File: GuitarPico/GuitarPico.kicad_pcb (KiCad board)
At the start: 2 copper layers, 100 x 100 mm, 132 parts, among them J1 INPUT, J2 INPUT, J3 OUTPUT, J4 OUTPUT, J5 Barrel_Jack_Switch, J6 VGA, J8 INPUT, J9 INPUT, Q1 2N3904, Q2 2N3904, Q3 2N3904, SW1 SW_Push, SW2 SW_Push, SW3 SW_Push, SW4 SW_Push, SW5 SW_Push, U1 LM358, U2 LM358, U3 Pico, U4 LM7805_TO220, U5 TL431LP, U6 4051

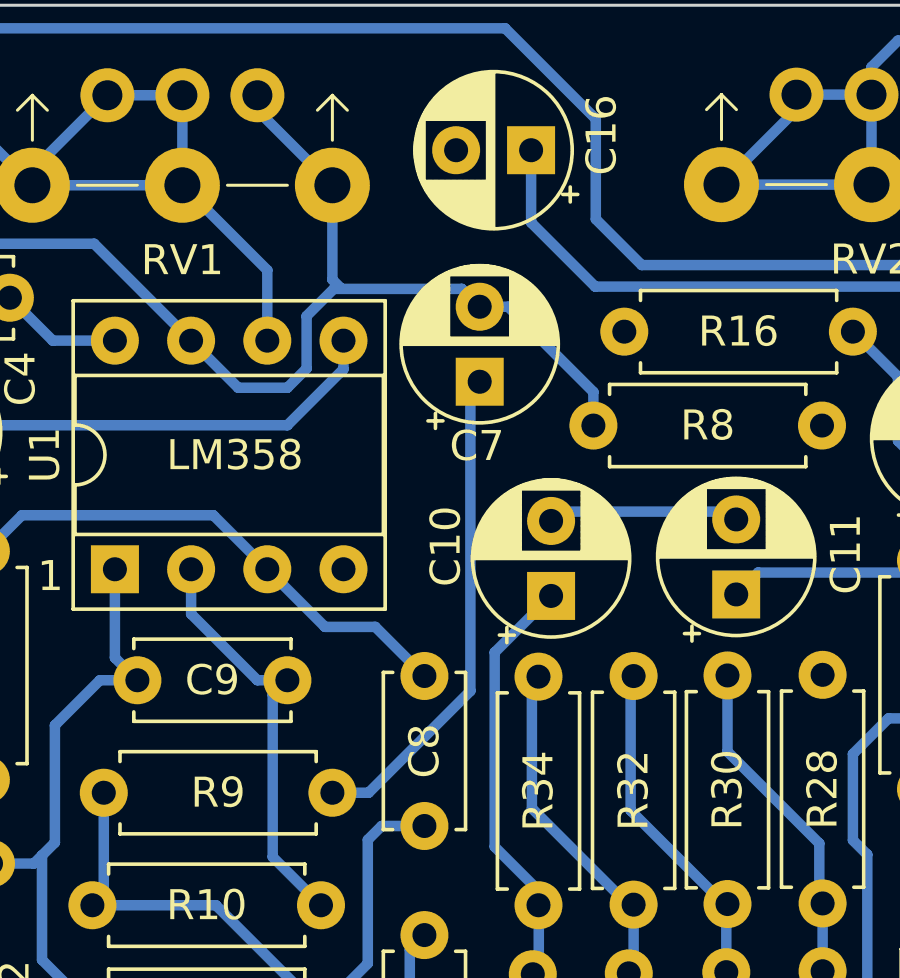
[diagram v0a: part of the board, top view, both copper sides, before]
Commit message: Minor code fixes
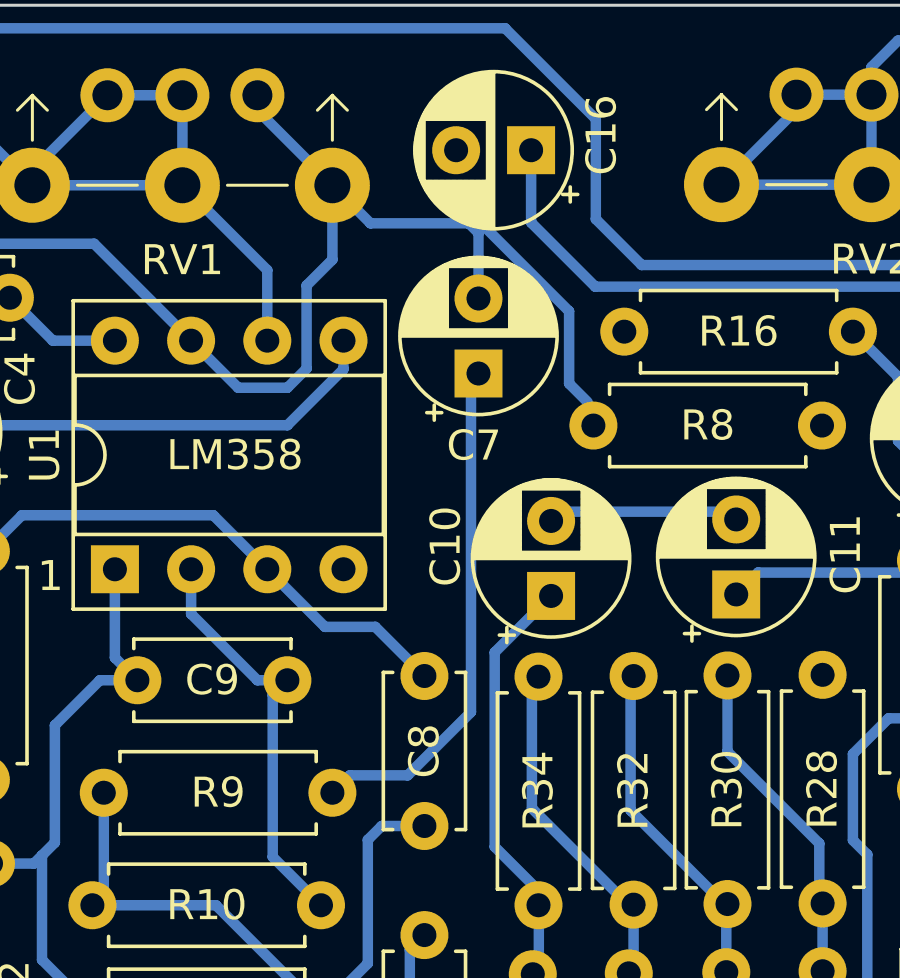
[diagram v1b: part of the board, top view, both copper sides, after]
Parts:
- moved C7 0.28 mm to (85.1, 72.3)
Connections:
- J2 pad G: unconnected-(J2-PadG) -> GND
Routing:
- net Net-(R7-Pad1): track 39.3 -> 42.2 mm
- net Net-(C7-Pad1): track 16.4 -> 17.0 mm
